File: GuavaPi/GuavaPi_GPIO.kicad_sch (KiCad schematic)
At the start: 1 part

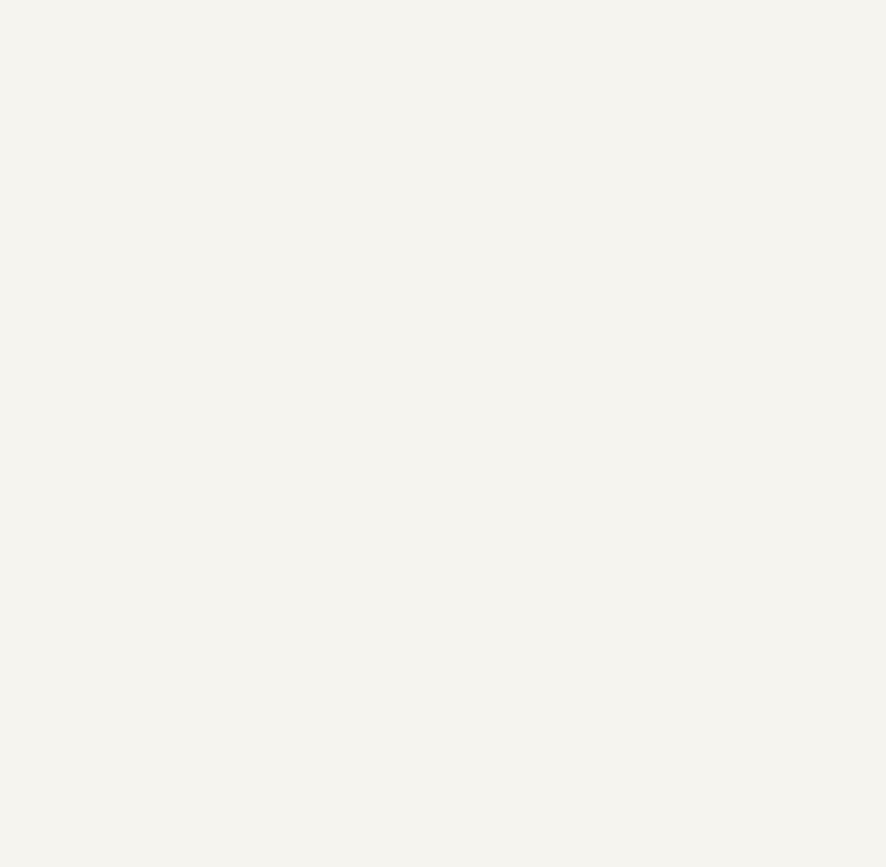
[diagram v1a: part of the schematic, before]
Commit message: Added EEMC
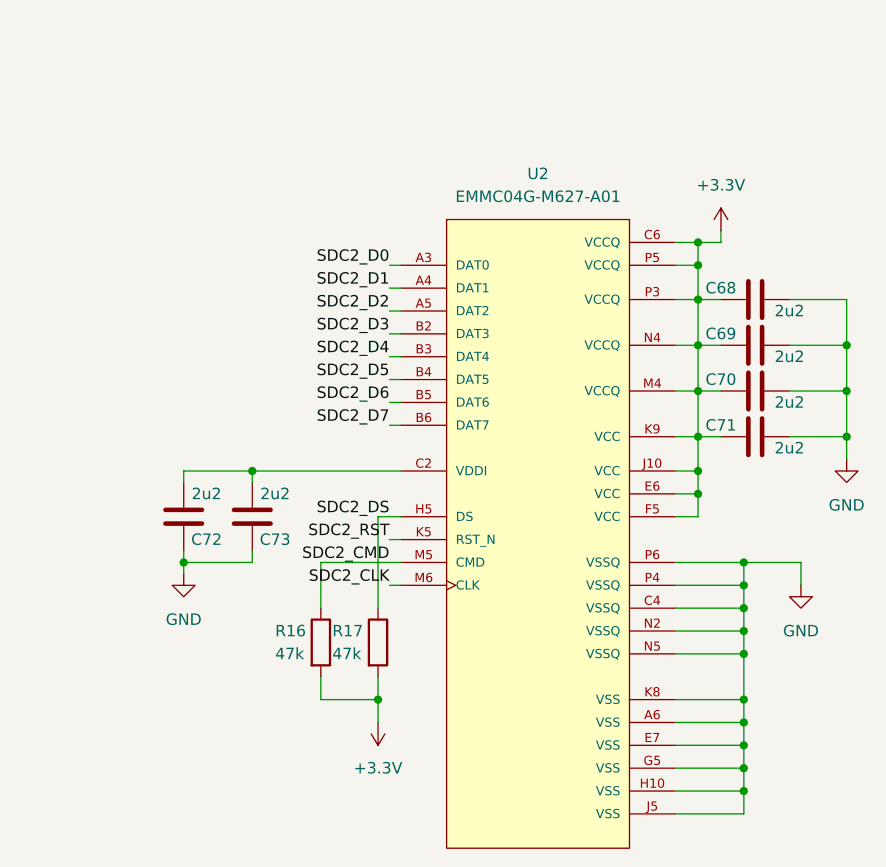
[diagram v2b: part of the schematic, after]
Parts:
- added C68, C69, C70, C71, C72, C73: 2u2, symbol Device:C
- added R16, R17: 47k, symbol Device:R
- added U2: EMMC04G-M627-A01, BGA153C50P14X14_1300X1150X100, symbol EMMC04G-M627-A01:EMMC04G-M627-A01
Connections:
- new net: C72.1, C73.1, U2.C2 (VDDI)
- new net +3.3V: C68.2, C69.2, C70.2, C71.2, R16.2, R17.2, U2.C6 (VCCQ), U2.E6 (VCC), U2.F5 (VCC), U2.J10 (VCC), U2.K9 (VCC), U2.M4 (VCCQ), U2.N4 (VCCQ), U2.P3 (VCCQ), U2.P5 (VCCQ)
- new net GND: C68.1, C69.1, C70.1, C71.1, C72.2, C73.2, U2.A6 (VSS), U2.C4 (VSSQ), U2.E7 (VSS), U2.G5 (VSS), U2.H10 (VSS), U2.J5 (VSS), U2.K8 (VSS), U2.N2 (VSSQ), U2.N5 (VSSQ), U2.P4 (VSSQ), U2.P6 (VSSQ)
- new net SDC2_CLK: U2.M6 (CLK)
- new net SDC2_CMD: R16.1, U2.M5 (CMD)
- new net SDC2_D0: U2.A3 (DAT0)
- new net SDC2_D1: U2.A4 (DAT1)
- new net SDC2_D2: U2.A5 (DAT2)
- new net SDC2_D3: U2.B2 (DAT3)
- new net SDC2_D4: U2.B3 (DAT4)
- new net SDC2_D5: U2.B4 (DAT5)
- new net SDC2_D6: U2.B5 (DAT6)
- new net SDC2_D7: U2.B6 (DAT7)
- new net SDC2_DS: R17.1, U2.H5 (DS)
- new net SDC2_RST: U2.K5 (RST_N)
